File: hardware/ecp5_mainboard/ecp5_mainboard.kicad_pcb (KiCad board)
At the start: 8 copper layers, 158.1 x 111.2 mm, 508 parts, among them J1 12V_EXT, J10 UART, J11 FLASH, J12 JTAG, J13 Micro_SD_Card, J2 USB_B_Micro, J3 HDMI_A, J4 USB_A, J5 EXT0, J6 EXT1, J7 EXT2, J8 EXT3, J9 PMOD_01, P1 SATA, P2 SATA, P3 PCIe_x4_EDGE, P4 JK0654219NL, Q1 BSH111BKR, Q2 BC850, Q3 BSH111BKR, Q4 BC850, Q5 BSH111BKR, Q6 BSH111BKR, Q7 BSH111BKR, Q8 BSH111BKR, Q9 BSH111BKR, SW1 CHP-081TA, SW2 SW_Push, SW3 SW_Push, SW4 SW_Push, SW5 SW_Push, SW6 SW_Push, U1 MAX811MEUS-T, U10 TPS62823, U12 93AA46B_OT, U13 FT2232H, U14 XUL535150.000JS6I8, U15 ECP5UM5G_85_CABGA756, U16 5P49V6965, U17 TPS2041B, U18 PCA9306, U19 TFP410, U2 LM3880, U20 TPS2041B, U21 KSZ9031RNXCA, U22 USB3300-EZK, U23 AS4C256M16D3, U24 AS4C256M16D3, U25 TPS51200DRC, U26 XL_XO_LVDS, U27 W25Q, U3 TLV75712PDR, U4 TPS565208, U5 LM21212-2, U6 TLV75712PDR, U7 TPS62823, U8 TPS62823, U9 TPS62823, X1 XO32, Y1 25MHz, Y2 25MHz, Y3 24MHz

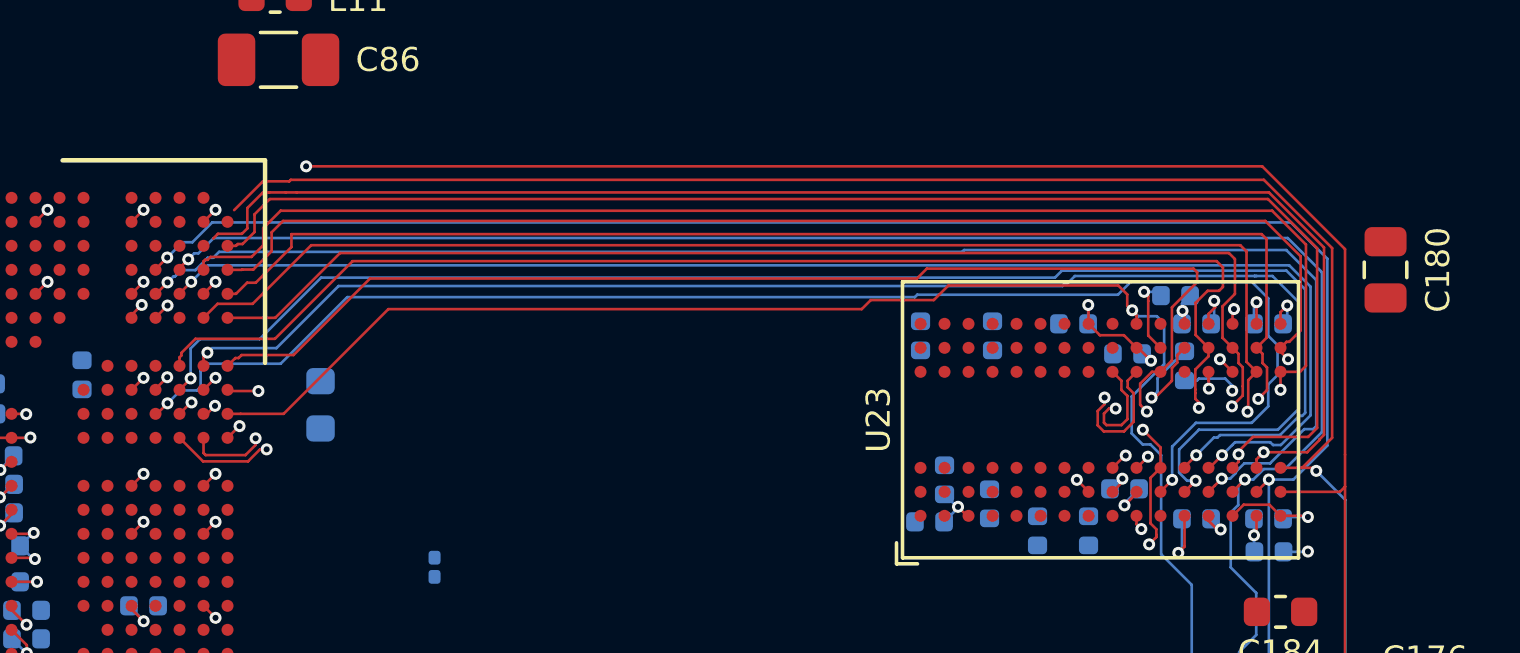
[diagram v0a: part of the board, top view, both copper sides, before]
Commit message: hardware/mainboard: DDR3 CA FPGA->chip0 length matching
Signed-off-by: David Shah <dave@ds0.me>
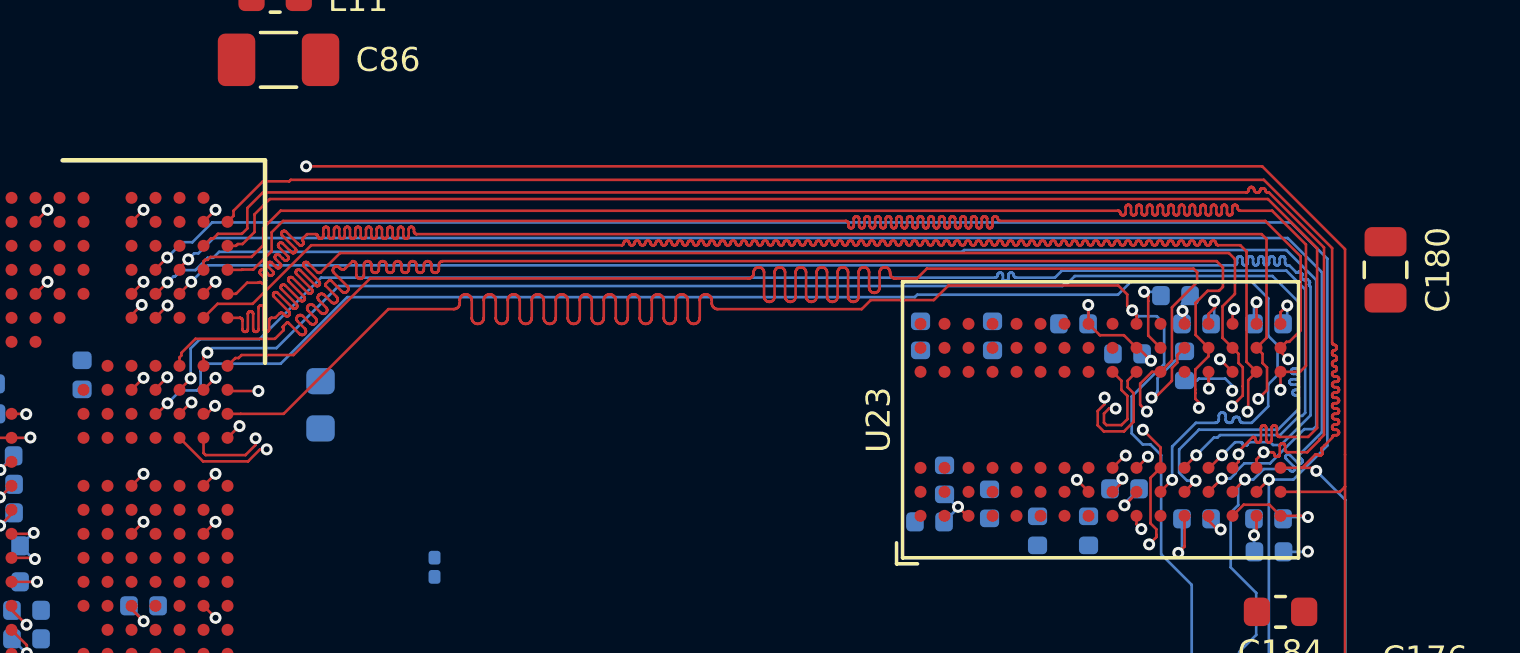
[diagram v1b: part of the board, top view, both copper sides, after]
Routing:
- net DDR3_CKE: track 67.0 -> 83.9 mm
- net DDR3_A10: track 68.6 -> 80.5 mm
- net DDR3_A4: track 67.6 -> 79.2 mm
- net DDR3_WE: track 66.4 -> 77.4 mm
- net DDR3_A6: track 66.3 -> 76.3 mm
- net DDR3_BA1: track 71.0 -> 80.6 mm
- net DDR3_A11: track 67.5 -> 76.9 mm
- net DDR3_CAS: track 68.0 -> 77.4 mm
- net DDR3_A8: track 67.0 -> 75.8 mm
- net DDR3_RAS: track 68.4 -> 75.3 mm
- net DDR3_A14: track 68.2 -> 74.2 mm
- net DDR3_A12: track 74.6 -> 79.0 mm
- net DDR3_A13: track 73.4 -> 76.4 mm
- net DDR3_A1: track 75.9 -> 78.9 mm
- net DDR3_A0: track 74.0 -> 76.6 mm
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
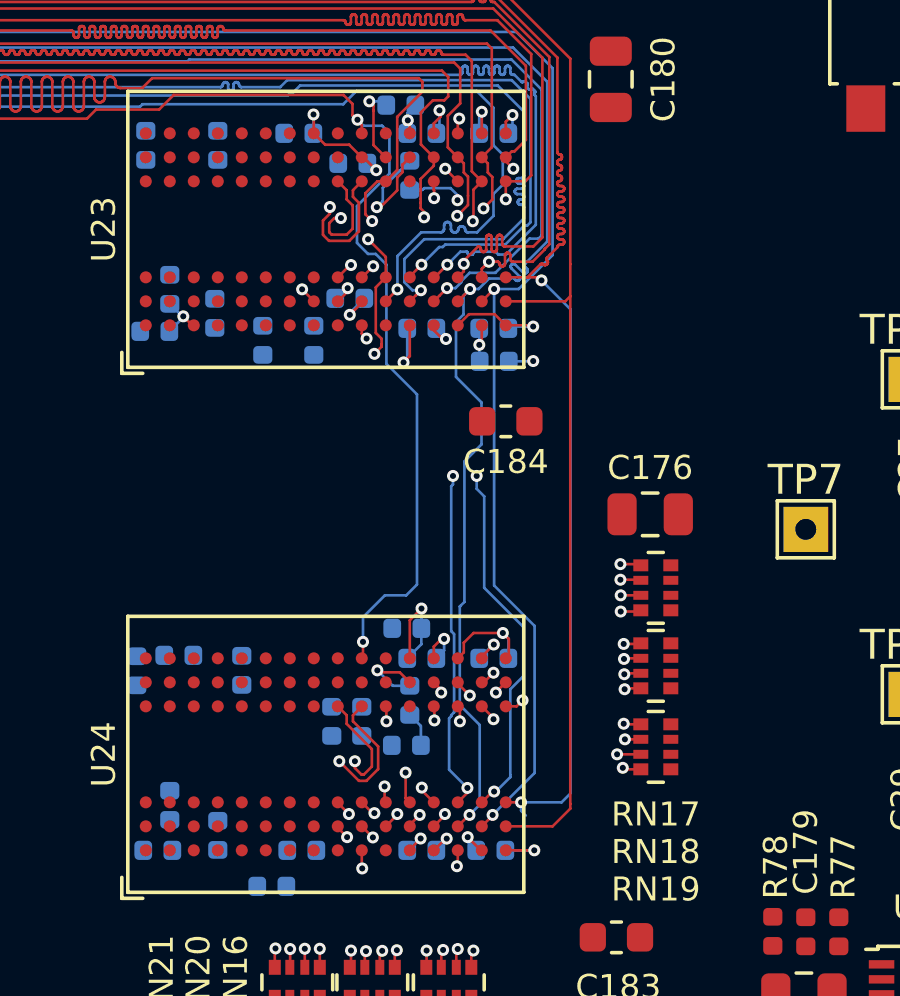
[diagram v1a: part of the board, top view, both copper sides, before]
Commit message: hardware/mainboard: DDR3 CA traces length matched with squiggly bois
Signed-off-by: David Shah <dave@ds0.me>
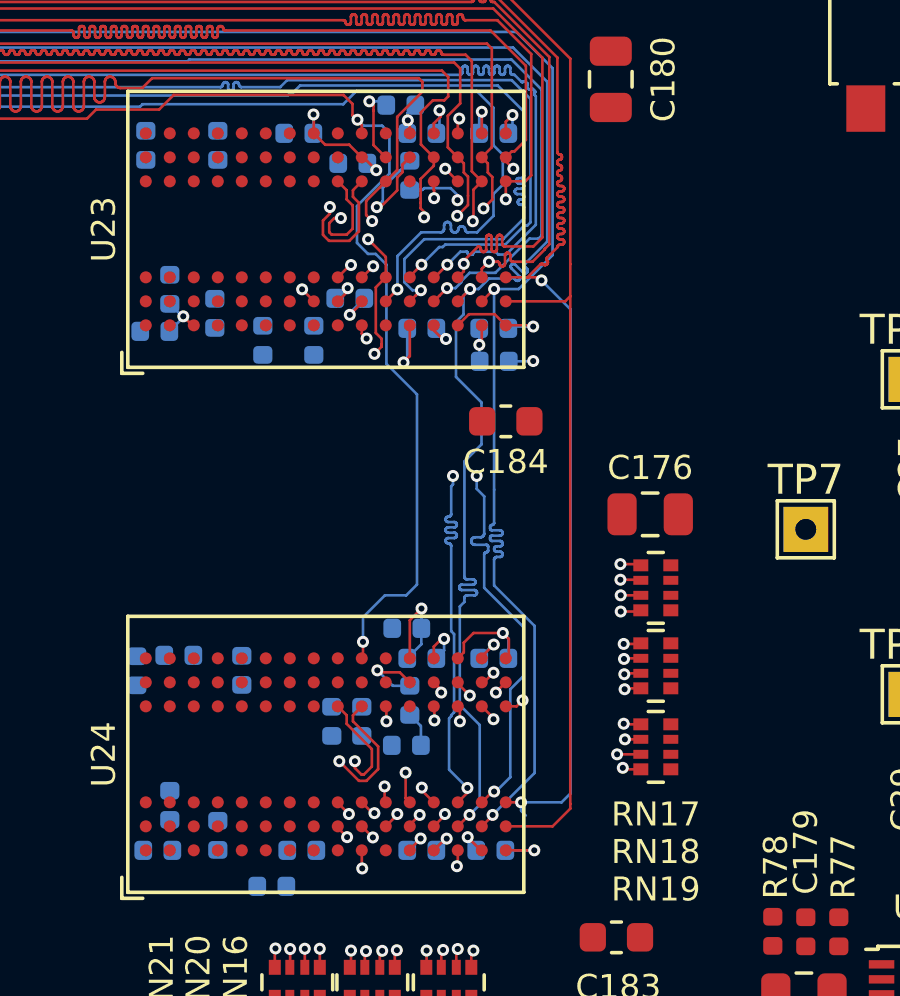
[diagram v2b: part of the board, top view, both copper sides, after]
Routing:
- net DDR3_A14: track 74.2 -> 77.0 mm
- net DDR3_WE: track 77.4 -> 80.0 mm
- net DDR3_CS: track 74.0 -> 76.2 mm
- net DDR3_A8: track 75.8 -> 77.5 mm
- net DDR3_A7: track 74.4 -> 76.2 mm
- net DDR3_A5: track 75.0 -> 76.6 mm
- net DDR3_A6: track 76.3 -> 77.9 mm
- net DDR3_A0: track 76.6 -> 78.1 mm
- net DDR3_ODT: track 71.9 -> 73.4 mm
- net DDR3_BA2: track 76.3 -> 77.8 mm
- net DDR3_A2: track 76.0 -> 77.4 mm
- net DDR3_RAS: track 75.3 -> 76.6 mm
- net DDR3_A11: track 76.9 -> 78.1 mm
- net DDR3_A3: track 75.4 -> 76.5 mm
- net DDR3_A9: track 76.2 -> 77.1 mm
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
